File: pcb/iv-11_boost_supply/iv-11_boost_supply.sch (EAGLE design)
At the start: 15 parts, among them IC1 LM555D, M1 IRF540NPBF

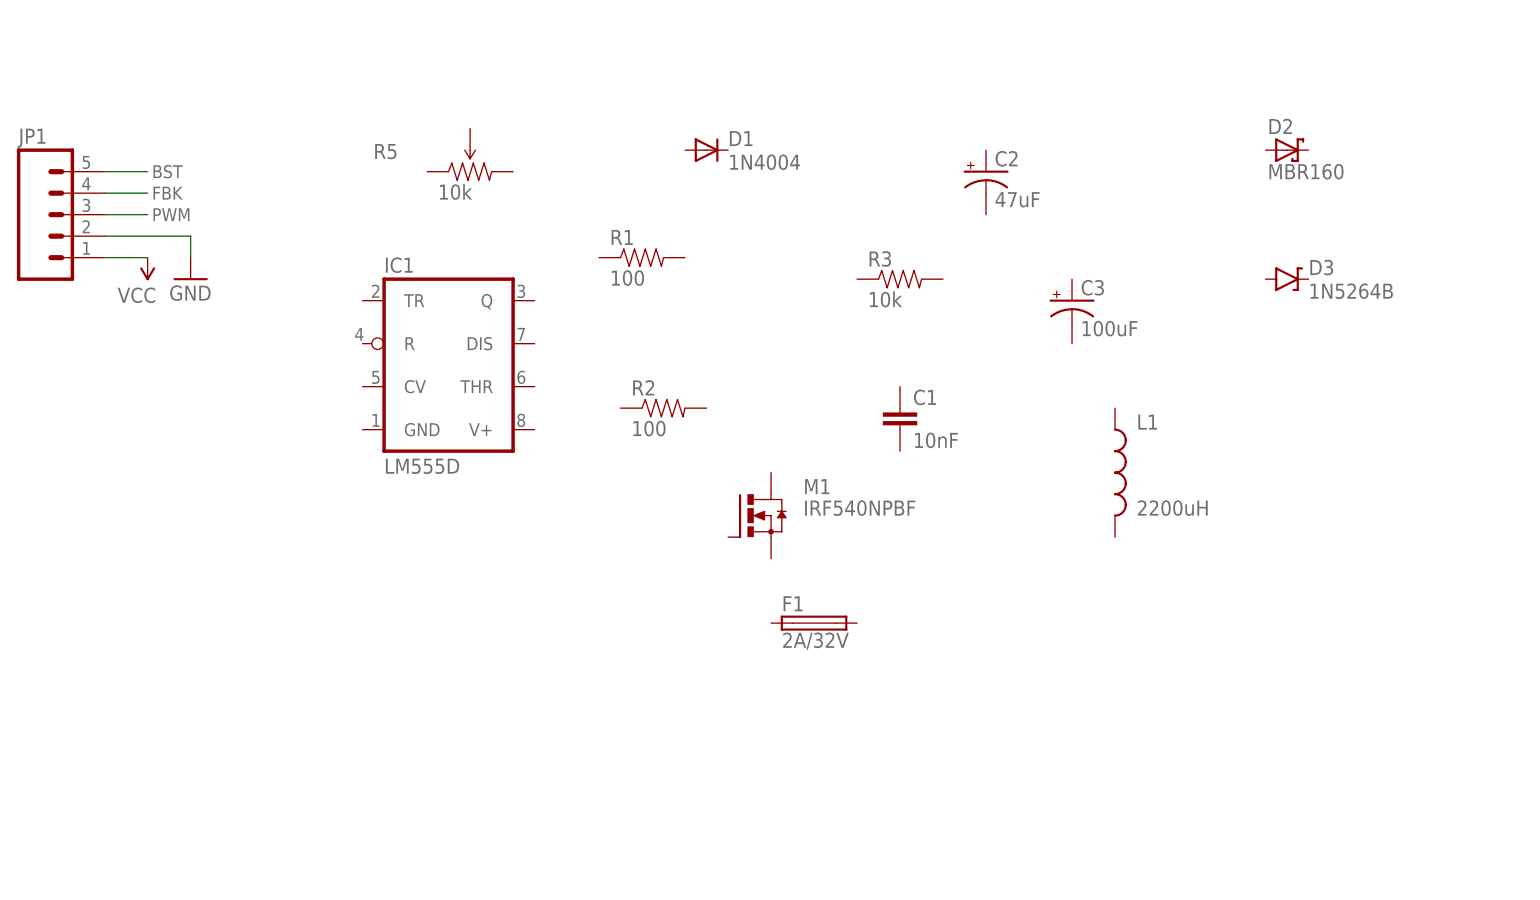
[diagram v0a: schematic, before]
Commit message: Did most of the board layout, found more parts to order
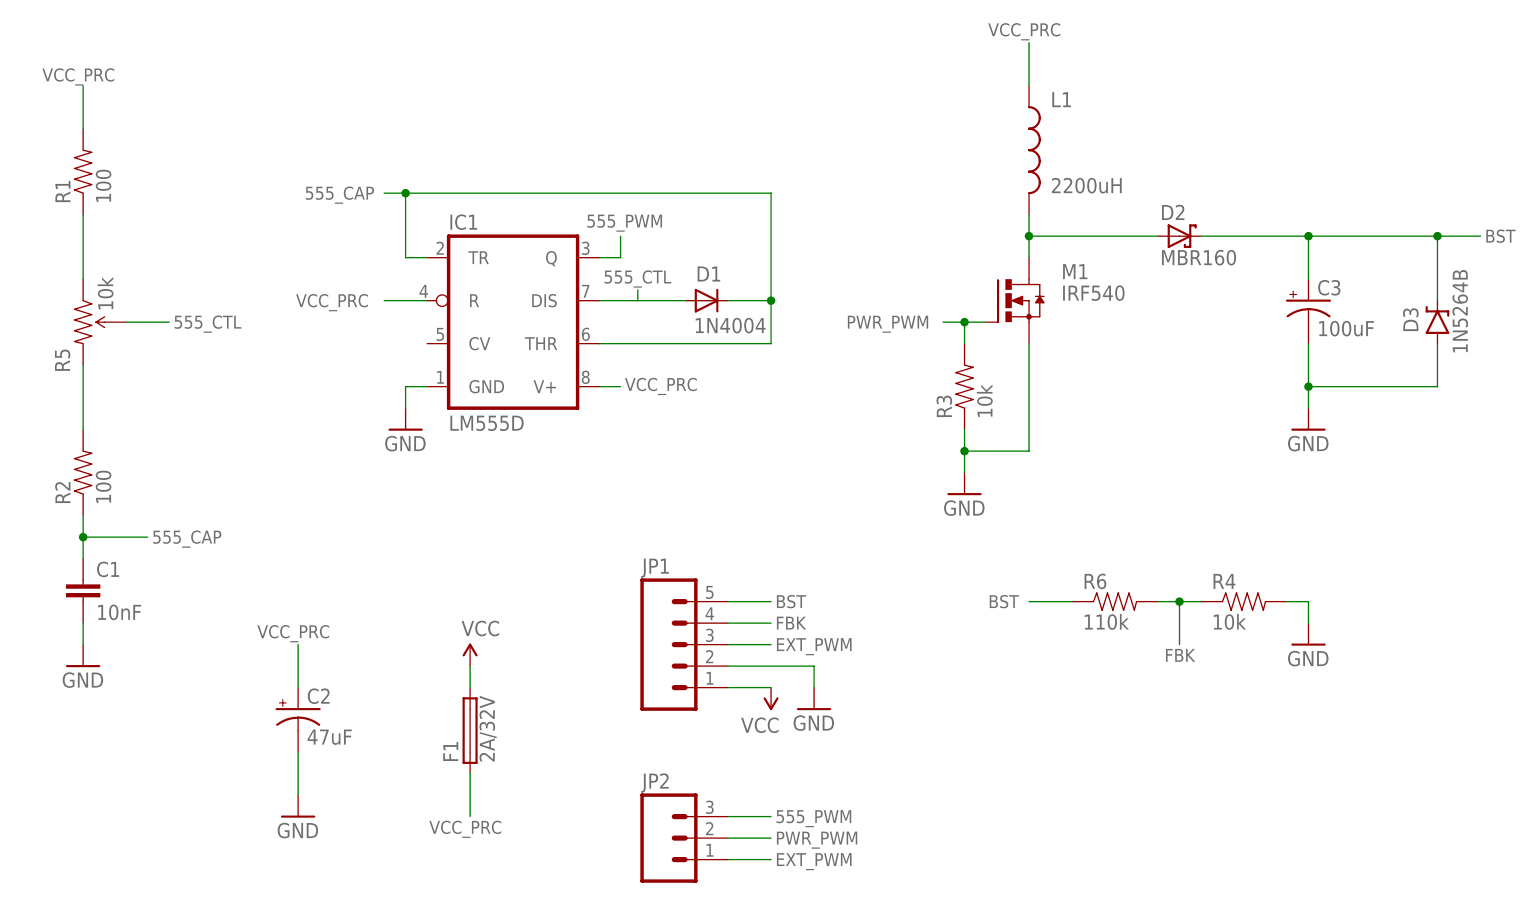
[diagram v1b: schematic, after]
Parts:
- added JP2: (no value), SparkFun-Connectors:M03LOCK
- added R4: 10k, SparkFun-Passives:RESISTOR1206
- added R6: 110k, SparkFun-Passives:RESISTOR1206
- D2: device adafruit:SCHOTTKY-DIODEDO201T15 -> adafruit:SCHOTTKY-DIODEDO35-7
- M1: value IRF540NPBF -> IRF540
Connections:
- removed net PWM: JP1.3
- new net 555_CAP: C1.1, D1.C, IC1.THR, IC1.TR, R2.1
- new net 555_CTL: D1.A, IC1.DIS, R5.WIPER
- new net 555_PWM: IC1.Q, JP2.3
- new net EXT_PWM: JP1.3, JP2.1
- new net N$1: R1.1, R5.CCW
- new net N$2: R2.2, R5.CW
- new net N$4: D2.A, L1.2, M1.D
- new net PWR_PWM: JP2.2, M1.G, R3.2
- new net VCC_PRC: C2.+, F1.1, IC1.R, IC1.V+, L1.1, R1.2
- net BST: now also C3.+, D2.C, D3.C, R6.1
- net FBK: now also R4.1, R6.2
- net GND: now also C1.2, C2.-, C3.-, D3.A, IC1.GND, M1.S, R3.1, R4.2
- net VCC: now also F1.2
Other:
- moved on the sheet: C1, C2, C3, D1, D2, D3, F1, IC1, JP1, L1, M1, R1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
